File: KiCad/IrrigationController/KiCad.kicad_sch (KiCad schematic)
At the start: 112 parts, among them IC1 MCP23017-E_SO, IC2 MCP23017-E_SO, IC3 DS89C21TMX_NOPB, J1 Screw_Terminal_01x03, J10 Screw_Terminal_01x05, J11 Screw_Terminal_01x02, J12 Screw_Terminal_01x02, J13 Screw_Terminal_01x04, J14 Screw_Terminal_01x02, J15 Screw_Terminal_01x02, J16 Screw_Terminal_01x02, J17 Screw_Terminal_01x02, J18 Screw_Terminal_01x02, J19 Screw_Terminal_01x02, J2 Screw_Terminal_01x03, J20 Screw_Terminal_01x05, J3 Screw_Terminal_01x03, J5 Screw_Terminal_01x03, J6 Screw_Terminal_01x02, J7 Screw_Terminal_01x02, J8 Screw_Terminal_01x02, J9 Screw_Terminal_01x02, K1 2071556-9, K2 2071556-9, Q1 2N3906, Q11 2N3904, Q12 2N3904, Q2 2N3906, Q3 2N3906, Q6 2N3904, Q7 2N3904, Q8 2N3904, SW1 SW_Push, U1 L298HN, U2 ARDUINO_MKR_WAN_1310, U3 L298HN, U4 L298HN, U5 L298HN, U7 L7805

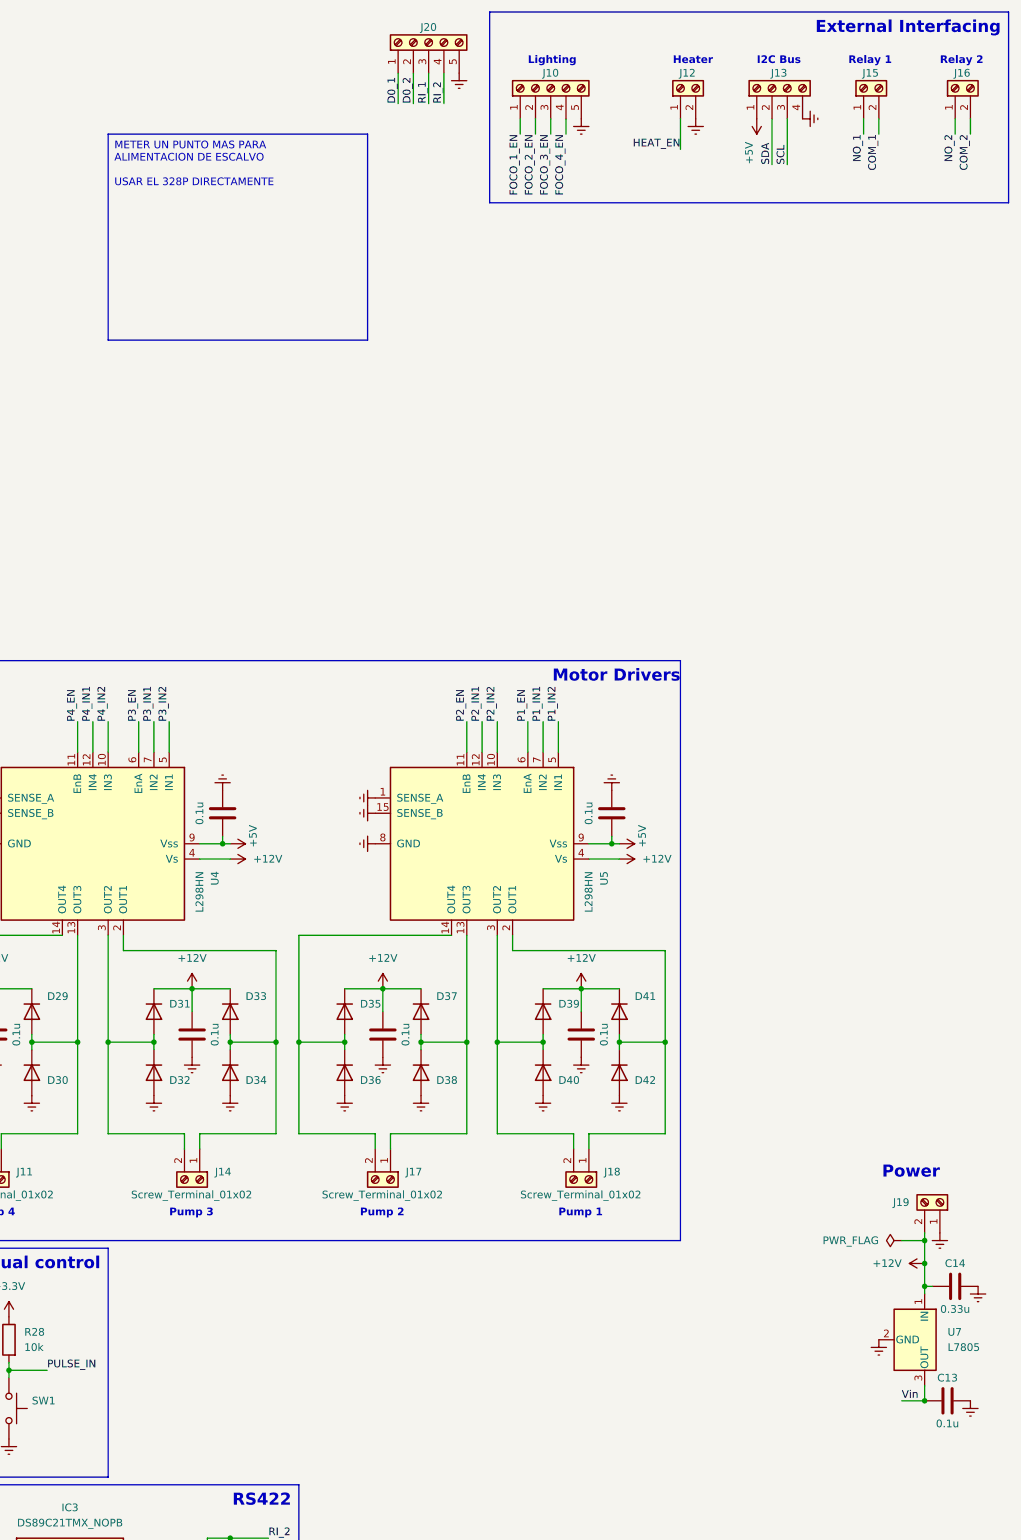
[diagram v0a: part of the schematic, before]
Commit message: tarjeta externa añadido
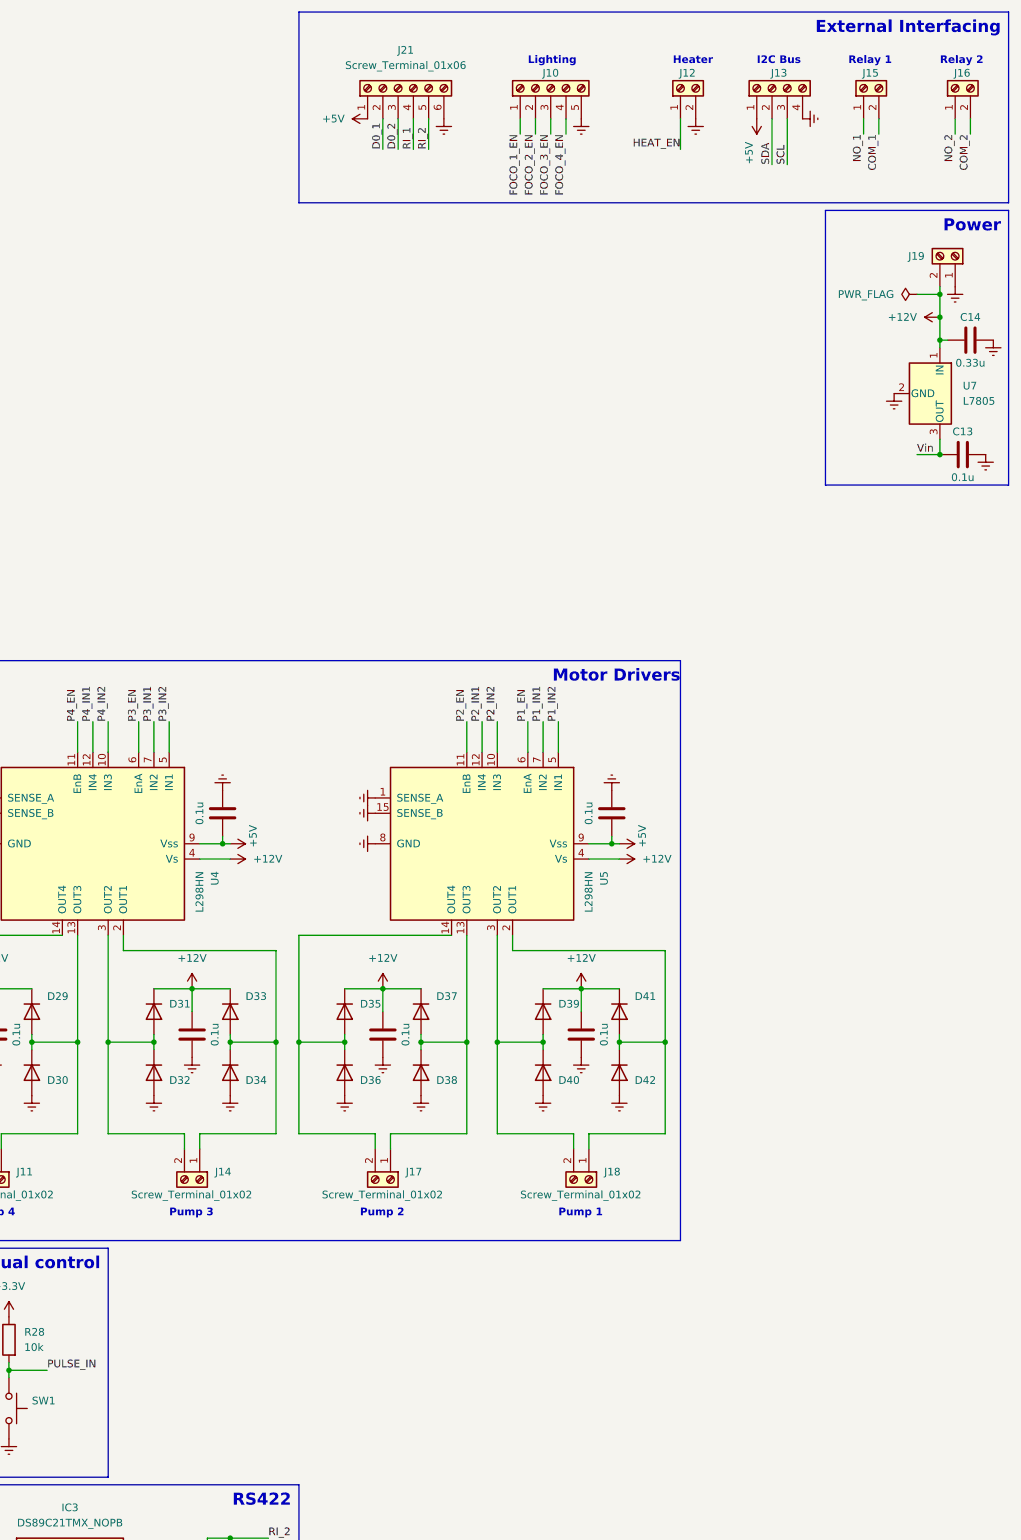
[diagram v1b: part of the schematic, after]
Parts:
- removed J20: Screw_Terminal_01x05, TerminalBlock_Phoenix:TerminalBlock_Phoenix_MKDS-1,5-5_1x05_P5.00mm_Horizontal, symbol Connector:Screw_Terminal_01x05
- added J21: Screw_Terminal_01x06, symbol Connector:Screw_Terminal_01x06
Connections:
- net +5V: now also J21.1 (Pin_1)
- net D0_1: now also J21.2 (Pin_2)
- net D0_2: now also J21.3 (Pin_3)
- net Earth: now also J21.6 (Pin_6)
- net RI_1: now also J21.4 (Pin_4)
- net RI_2: now also J21.5 (Pin_5)
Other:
- moved on the sheet: C13, C14, J19, U7

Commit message: qwer
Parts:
- Q3: Ref Mouser (none) -> 637-2N3906
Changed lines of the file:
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@@
       (effects (font (size 1.27 1.27)) (justify left) hide)
+    )
+    (property "Ref Mouser" "637-2N3906" (at 31.75 143.51 0)
+      (effects (font (size 1.27 1.27)) hide)
     )
     (pin "1")
